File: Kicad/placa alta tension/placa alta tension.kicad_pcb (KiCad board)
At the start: 2 copper layers, 60 x 80 mm, 33 parts, among them J1 Conn_01x05_Socket, J2 Screw_Terminal_01x02, J3 Screw_Terminal_01x02, J4 Screw_Terminal_01x02, Q2 2N7000, Q4 2N7000, U1 MOC3023M, U2 4N25, U3 MOC3023M

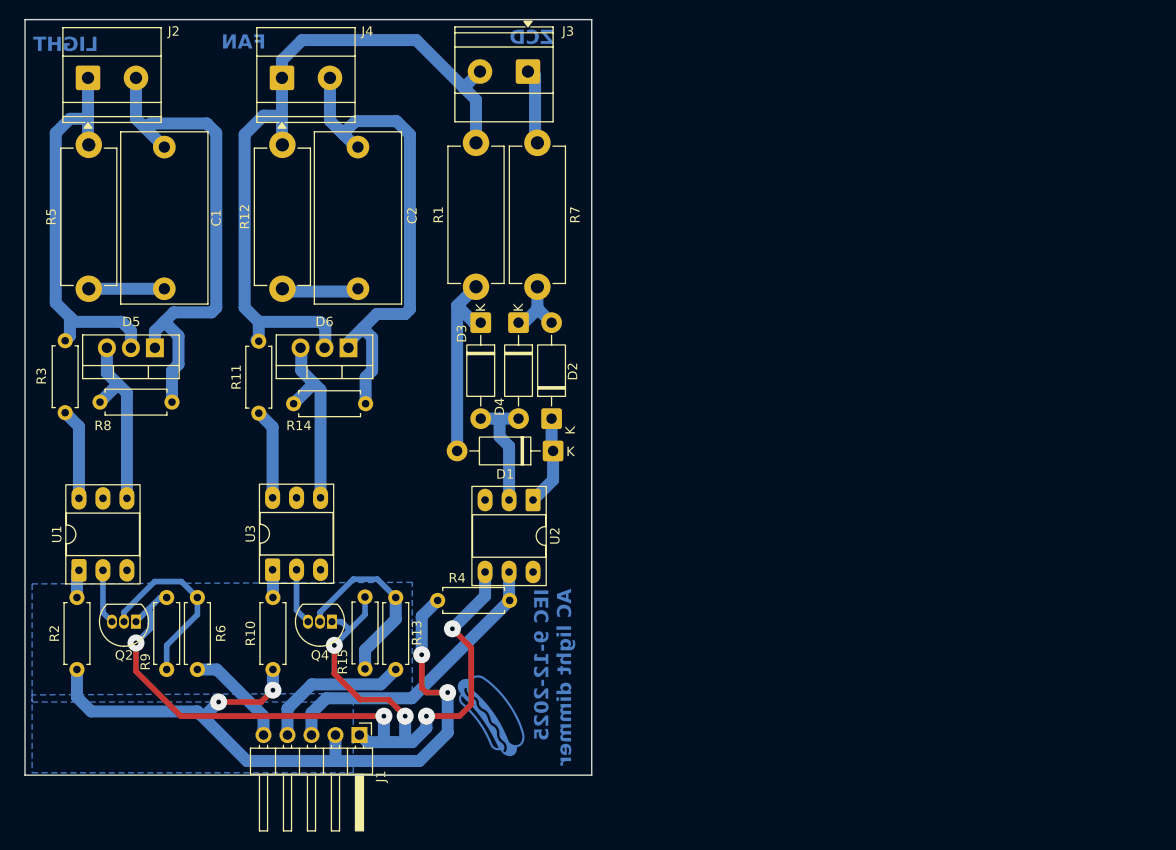
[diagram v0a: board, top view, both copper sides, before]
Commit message: placa v2
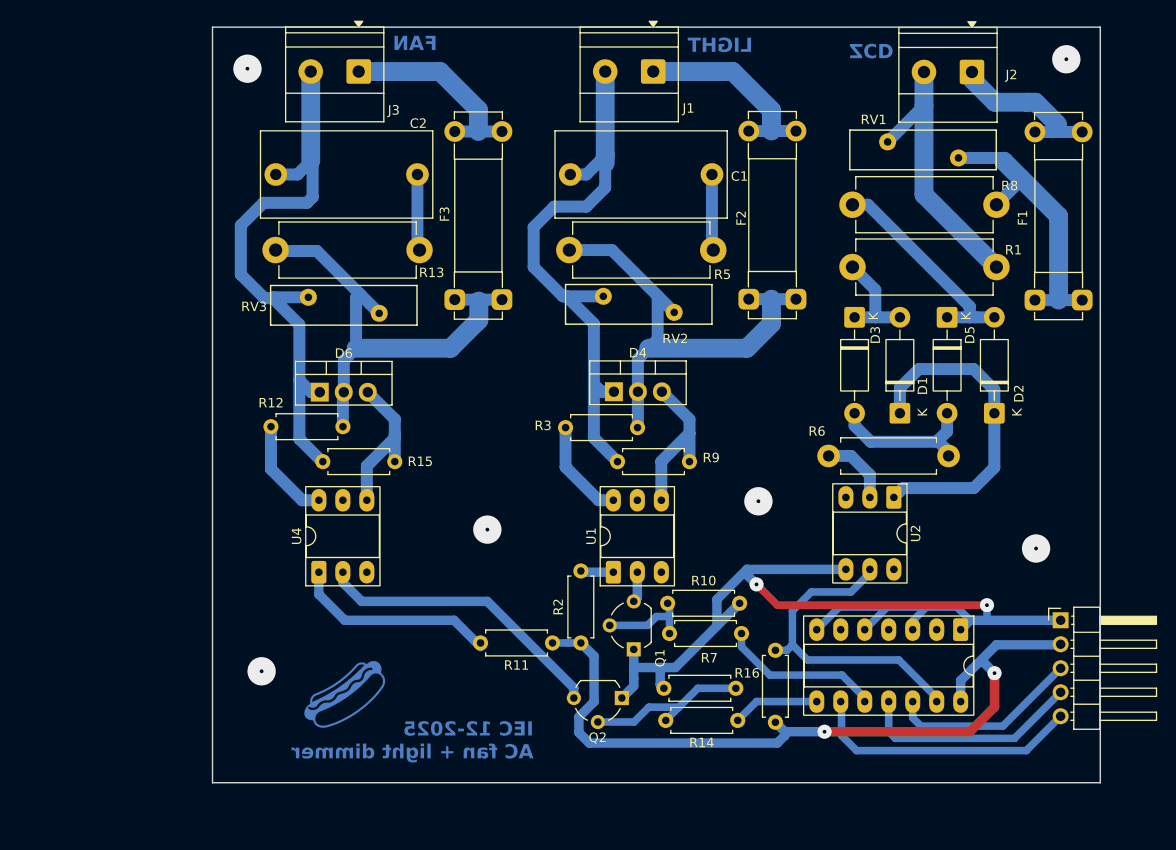
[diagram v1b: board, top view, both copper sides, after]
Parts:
- removed Q4: 2N7000, Package_TO_SOT_THT:TO-92_Inline
- added F1: Fuse, Fuse:Fuseholder_Clip-5x20mm_Bel_FC-203-22_Lateral_P17.80x5.00mm_D1.17mm_Horizontal, F.Cu at (201.7, 80.7)
- added F2: Fuse, Fuse:Fuseholder_Clip-5x20mm_Bel_FC-203-22_Lateral_P17.80x5.00mm_D1.17mm_Horizontal, F.Cu at (171.4, 80.6)
- added F3: Fuse, Fuse:Fuseholder_Clip-5x20mm_Bel_FC-203-22_Lateral_P17.80x5.00mm_D1.17mm_Horizontal, F.Cu at (140.2, 80.7)
- added Q1: 2N7000, Package_TO_SOT_THT:TO-92_Wide, F.Cu at (159.2, 117.7)
- added R16: 1M, Resistor_THT:R_Axial_DIN0207_L6.3mm_D2.5mm_P7.62mm_Horizontal, F.Cu at (170.0, 121.8)
- added RV1: Varistor, Varistor:RV_Disc_D15.5mm_W4.2mm_P7.5mm, F.Cu at (186.1, 64.0)
- added RV2: Varistor, Varistor:RV_Disc_D15.5mm_W4.2mm_P7.5mm, F.Cu at (163.5, 82.0)
- added RV3: Varistor, Varistor:RV_Disc_D15.5mm_W4.2mm_P7.5mm, F.Cu at (132.2, 82.1)
- added U4: MOC3023M, Package_DIP:DIP-6_W7.62mm_Socket_LongPads, F.Cu at (125.9, 109.5)
- D4: value 1N4007 -> Generic_Triac_A1A2G; footprint Diode_THT:D_DO-41_SOD81_P10.16mm_Horizontal -> Package_TO_SOT_THT:TO-220-3_Vertical
- D5: value Generic_Triac_A1A2G -> 1N4007; footprint Package_TO_SOT_THT:TO-220-3_Vertical -> Diode_THT:D_DO-41_SOD81_P10.16mm_Horizontal
- J1: value Conn_01x05_Socket -> Screw_Terminal_01x02; footprint Connector_PinHeader_2.54mm:PinHeader_1x05_P2.54mm_Horizontal -> TerminalBlock_Phoenix:TerminalBlock_Phoenix_MKDS-1,5-2-5.08_1x02_P5.08mm_Horizontal
- J4: value Screw_Terminal_01x02 -> Conn_01x05_Socket; footprint TerminalBlock_Phoenix:TerminalBlock_Phoenix_MKDS-1,5-2-5.08_1x02_P5.08mm_Horizontal -> Connector_PinHeader_2.54mm:PinHeader_1x05_P2.54mm_Horizontal
- Q2: footprint Package_TO_SOT_THT:TO-92_Inline -> Package_TO_SOT_THT:TO-92_Wide
- R1: value 18k -> 10k
- R10: value 180 -> 1M
- R11: value 220 -> 180
- R12: value 2.4k -> 220; footprint Resistor_THT:R_Axial_DIN0614_L14.3mm_D5.7mm_P15.24mm_Horizontal -> Resistor_THT:R_Axial_DIN0207_L6.3mm_D2.5mm_P7.62mm_Horizontal
- R13: value 5 -> 2.4k; footprint Resistor_THT:R_Axial_DIN0207_L6.3mm_D2.5mm_P7.62mm_Horizontal -> Resistor_THT:R_Axial_DIN0614_L14.3mm_D5.7mm_P15.24mm_Horizontal
- R14: value 220 -> 5
- R15, R9: value 1M -> 220
- R6: value 5 -> 2k; footprint Resistor_THT:R_Axial_DIN0207_L6.3mm_D2.5mm_P7.62mm_Horizontal -> Resistor_THT:R_Axial_DIN0411_L9.9mm_D3.6mm_P12.70mm_Horizontal
- R7: value 18k -> 5; footprint Resistor_THT:R_Axial_DIN0614_L14.3mm_D5.7mm_P15.24mm_Horizontal -> Resistor_THT:R_Axial_DIN0207_L6.3mm_D2.5mm_P7.62mm_Horizontal
- R8: value 220 -> 10k; footprint Resistor_THT:R_Axial_DIN0207_L6.3mm_D2.5mm_P7.62mm_Horizontal -> Resistor_THT:R_Axial_DIN0614_L14.3mm_D5.7mm_P15.24mm_Horizontal
- U3: value MOC3023M -> 74HC14; footprint Package_DIP:DIP-6_W7.62mm_Socket_LongPads -> Package_DIP:DIP-14_W7.62mm_Socket_LongPads
- moved J4 100.5 mm to (204.4, 114.6)
- moved J2 93.6 mm to (195.0, 56.5), turned to 180 degrees
- moved D5 83.9 mm to (192.4, 82.5), turned to -90 degrees
- moved R8 82.4 mm to (182.4, 70.6)
- moved J1 76.8 mm to (161.3, 56.5), turned to 180 degrees
- moved U3 73.1 mm to (193.8, 115.6), turned to -90 degrees
- moved R6 70.6 mm to (179.8, 97.2), turned to 0 degrees
- moved R5 66.2 mm to (167.6, 75.4), turned to 180 degrees
- moved R9 59.6 mm to (165.1, 97.8), turned to 180 degrees
- moved C1 59.2 mm to (167.5, 67.4), turned to 180 degrees
- moved R14 57.8 mm to (170.2, 125.2), turned to 180 degrees
- moved U1 56.6 mm to (157.0, 109.5)
- moved R2 53.4 mm to (153.6, 117.0)
- moved R3 53.0 mm to (152.0, 94.2), turned to 0 degrees
- moved Q2 52.1 mm to (157.9, 122.8)
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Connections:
- C1 pad 2: Net-(D5-A1) -> /HV11
- D2 pad 2: Net-(D2-A) -> /HV9
- D4 pad 1: Net-(D2-A) -> /HV11
- D4 pad 2: Net-(D3-A) -> Net-(D4-A2)
- D5 pad 1: Net-(D5-A1) -> /HV9
- D5 pad 2: LIGHT_LINE -> Net-(D3-A)
- D6 pad 2: DIMMING_LINE -> Net-(D6-A2)
- J1 pad 1: GND -> LIGHT_LINE
- J1 pad 2: +5V -> /HV11
- J2 pad 1: LIGHT_LINE -> Net-(J2-Pin_1)
- J2 pad 2: Net-(D5-A1) -> Net-(J2-Pin_2)
- J3 pad 1: N -> DIMMING_LINE
- J3 pad 2: DIMMING_LINE -> Net-(D6-A1)
- J4 pad 1: DIMMING_LINE -> GND
- J4 pad 2: Net-(D6-A1) -> +5V
- R1 pad 2: DIMMING_LINE -> Net-(J2-Pin_2)
- R10 pad 1: +5V -> Net-(Q1-G)
- R10 pad 2: Net-(R10-Pad2) -> GND
- R11 pad 1: Net-(R11-Pad1) -> +5V
- R11 pad 2: DIMMING_LINE -> Net-(R11-Pad2)
- R12 pad 1: Net-(C2-Pad1) -> Net-(R12-Pad1)
- R12 pad 2: DIMMING_LINE -> Net-(D6-A2)
- R13 pad 1: /FAN -> Net-(C2-Pad1)
- R13 pad 2: Net-(Q4-G) -> Net-(D6-A2)
- R14 pad 1: Net-(D6-G) -> Net-(R14-Pad1)
- R14 pad 2: Net-(D6-A1) -> Net-(Q2-G)
- R15 pad 1: Net-(Q4-G) -> Net-(D6-G)
- R15 pad 2: GND -> Net-(D6-A1)
- R3 pad 2: LIGHT_LINE -> Net-(D4-A2)
- R4 pad 2: /ZCD -> Net-(R4-Pad2)
- R5 pad 2: LIGHT_LINE -> Net-(D4-A2)
- R6 pad 1: /LIGHT -> Net-(R6-Pad1)
- R6 pad 2: Net-(Q2-G) -> Net-(D3-A)
- R7 pad 1: Net-(D2-A) -> Net-(R7-Pad1)
- R7 pad 2: N -> Net-(Q1-G)
- R8 pad 1: Net-(D5-G) -> /HV9
- R8 pad 2: Net-(D5-A1) -> N
- R9 pad 1: Net-(Q2-G) -> Net-(D4-G)
- R9 pad 2: GND -> /HV11
- U1 pad 2: Net-(Q2-D) -> Net-(Q1-D)
- U1 pad 4: Net-(D5-G) -> Net-(D4-G)
- U2 pad 2: Net-(D3-A) -> Net-(R6-Pad1)
- U2 pad 5: /ZCD -> Net-(R4-Pad2)
- U3 pad 1: Net-(R10-Pad2) -> GND
- U3 pad 2: Net-(Q4-D) -> unconnected-(U3-Pad2)
- U3 pad 3: unconnected-(U3-NC-Pad3) -> GND
- U3 pad 4: Net-(D6-G) -> unconnected-(U3-Pad4)
- U3 pad 5: unconnected-(U3-NC-Pad5) -> GND
- U3 pad 6: Net-(R11-Pad1) -> unconnected-(U3-Pad6)
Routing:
- net /HV11: track 0.00 -> 61.2 mm
- net DIMMING_LINE: track 78.5 -> 21.6 mm
- net Net-(D5-A1): track 53.8 -> 0.00 mm
- net Net-(D4-A2): track 0.00 -> 50.3 mm
- net Net-(D6-A2): track 0.00 -> 49.9 mm
- net Net-(R4-Pad2): track 0.00 -> 33.9 mm
- net Net-(J2-Pin_2): track 0.00 -> 29.6 mm
- net Net-(Q2-D): track 5.84 -> 31.2 mm
- net Net-(D1-K): track 9.56 -> 34.9 mm
- net N: track 8.29 -> 30.9 mm
- net /HV9: track 0.00 -> 21.8 mm
- net Net-(R11-Pad2): track 0.00 -> 21.8 mm
- net LIGHT_LINE: track 42.8 -> 21.4 mm
- net Net-(Q4-G): track 20.2 -> 0.00 mm
- net Net-(D5-G): track 19.7 -> 0.00 mm
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- removed copper zone on B.Cu, net GND
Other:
- board size 60 x 80 mm -> 94 x 80 mm
- board text added: "IEC 12-2025 AC fan + light dimmer"
- board text removed: "IEC 9-12-2025 AC light dimmer"
